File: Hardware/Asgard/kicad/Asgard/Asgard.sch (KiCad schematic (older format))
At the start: 10 parts

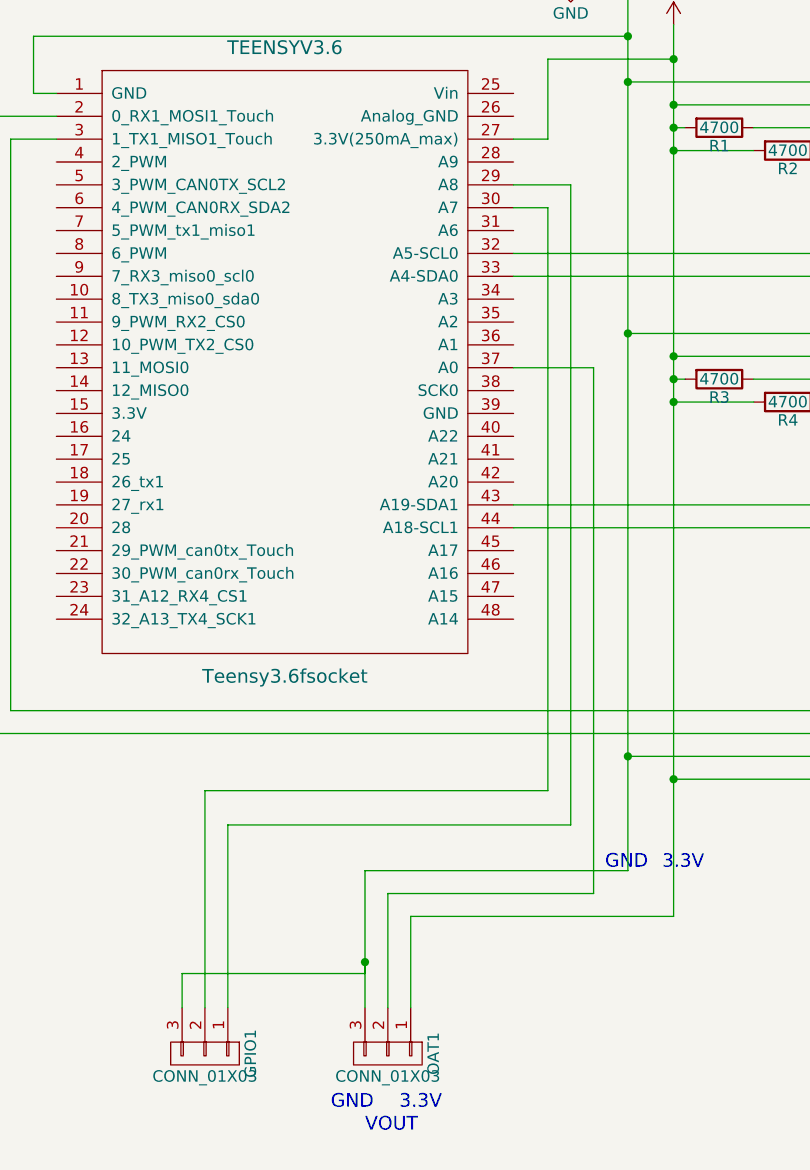
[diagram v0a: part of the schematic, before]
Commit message: PCB candidate 4
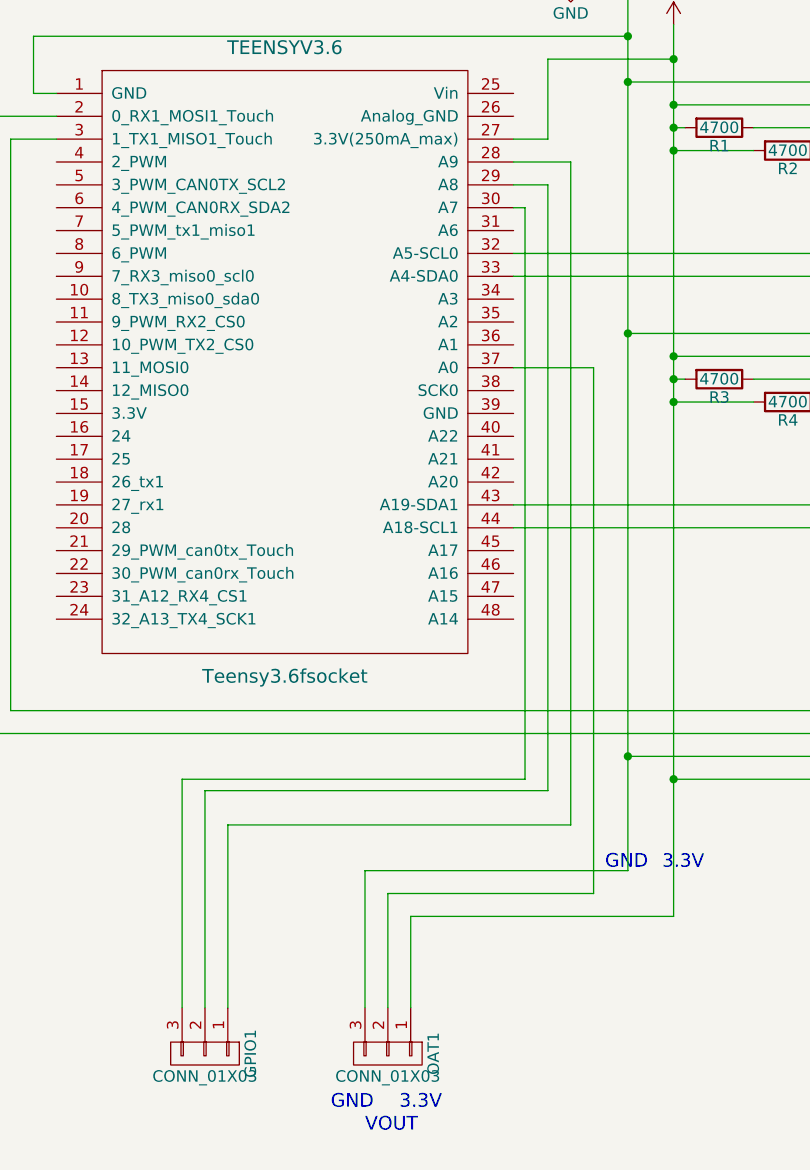
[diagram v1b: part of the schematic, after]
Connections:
- net GND: no longer GPIO1.3 (P3)
- net at TEENSYV3.6.28 (A9): now also GPIO1.1 (P1)
- net at TEENSYV3.6.29 (A8): now also GPIO1.2 (P2); no longer GPIO1.1 (P1)
- net at TEENSYV3.6.30 (A7): now also GPIO1.3 (P3); no longer GPIO1.2 (P2)
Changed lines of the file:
@@
 	4000 3350 3650 3350
 Wire Wire Line
-	3000 6150 3000 5550
-Wire Wire Line
-	3000 5550 4150 5550
+	4150 5550 3000 5550
 Wire Wire Line
 	4150 1600 3900 1600
@@
 $EndComp
 Wire Wire Line
-	2200 6150 2200 6000
-Wire Wire Line
-	2200 6000 3000 6000
-Wire Wire Line
-	3000 6000 3000 5950
-Connection ~ 3000 5950
+	2200 5150 2200 6150
 Wire Wire Line
 	3800 5200 2300 5200
@@
 	2400 6150 2400 5350
 Wire Wire Line
-	3900 5350 2400 5350
+	2400 5350 3900 5350
 Wire Wire Line
-	3900 2550 3900 5350
+	3900 5350 3900 2450
 Wire Wire Line
-	3800 5200 3800 2650
+	3800 2550 3800 5200
 Wire Wire Line
-	3800 2650 3650 2650
+	3900 2450 3650 2450
 Wire Wire Line
-	3900 2550 3650 2550
+	3800 2550 3650 2550
+Wire Wire Line
+	3000 5550 3000 6150
+Wire Wire Line
+	2200 5150 3700 5150
+Wire Wire Line
+	3700 5150 3700 2650
+Wire Wire Line
+	3700 2650 3650 2650
 $EndSCHEMATC
